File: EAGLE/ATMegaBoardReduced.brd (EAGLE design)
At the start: 55.9 x 50.5 mm, 18 parts, among them IC2 ATMEGA168-20P, IC3 REG1117, X1 49S/18PF

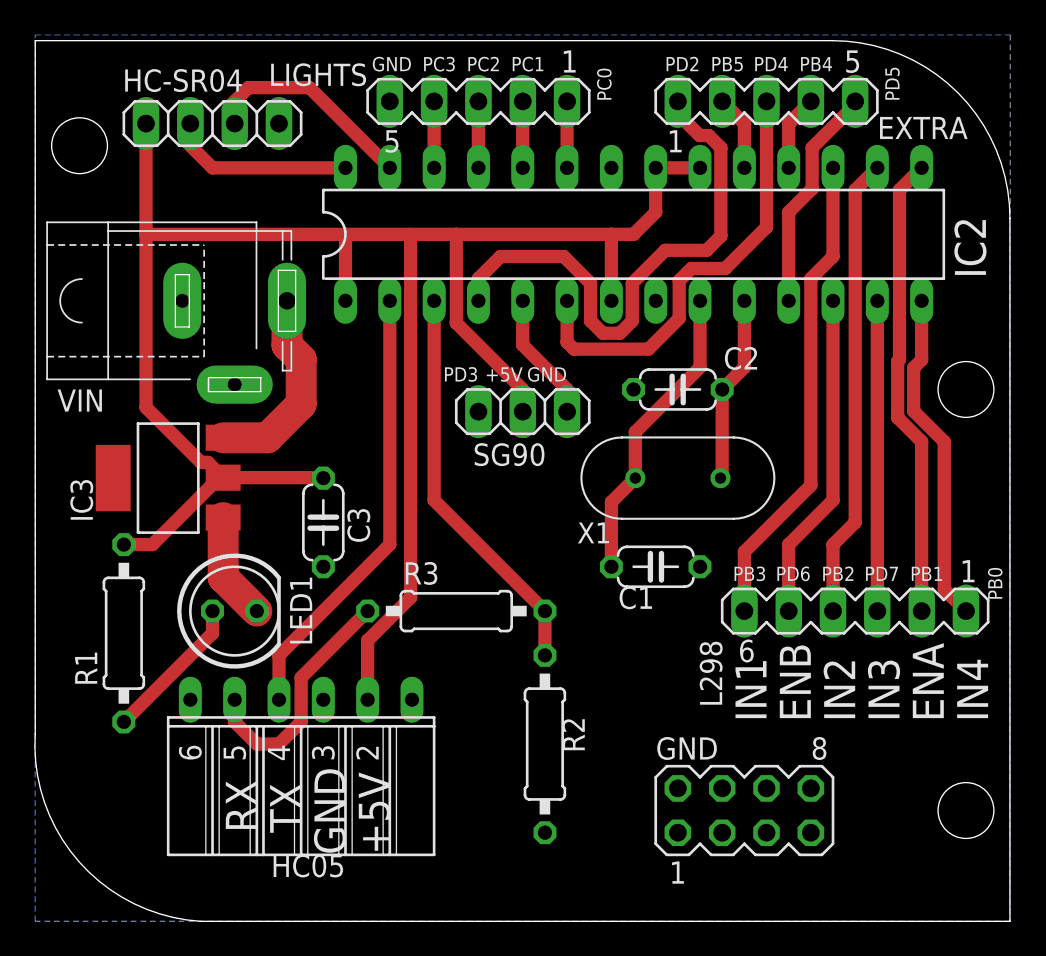
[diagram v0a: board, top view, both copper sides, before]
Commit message: minor board updates
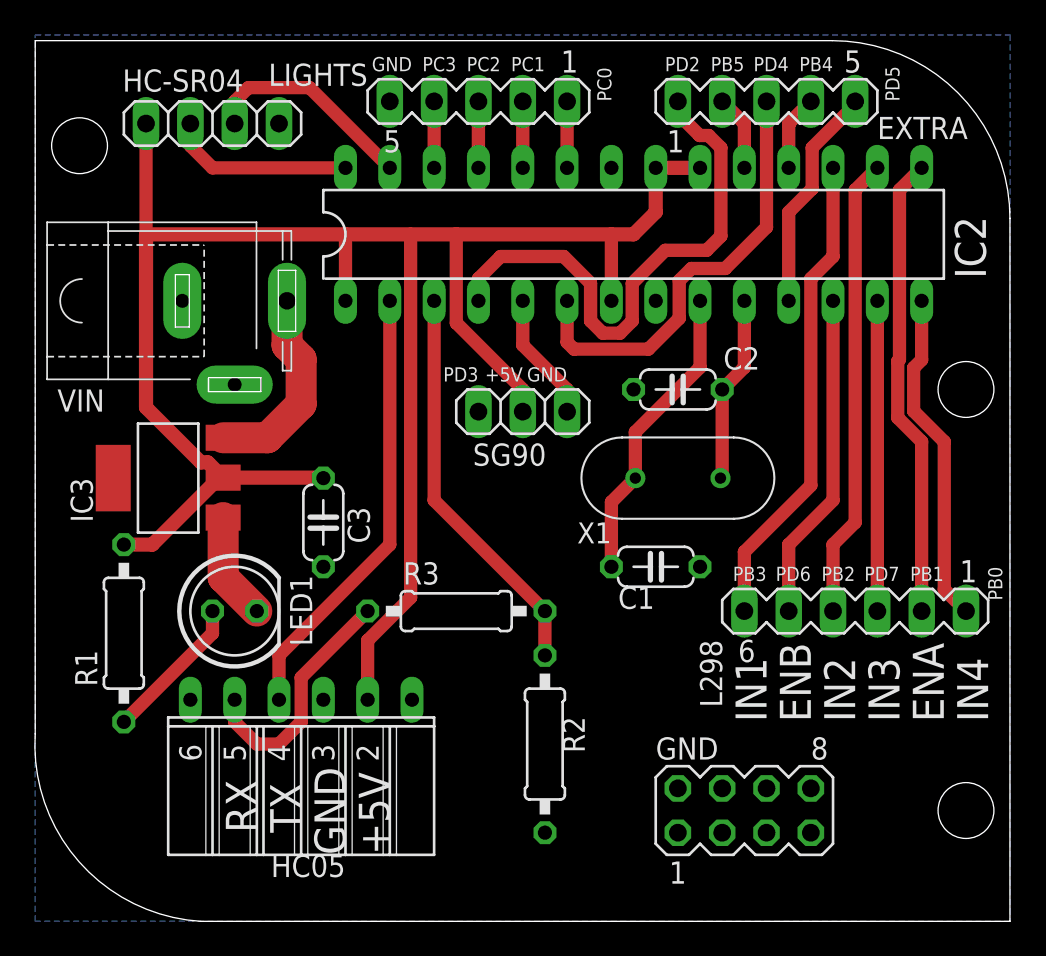
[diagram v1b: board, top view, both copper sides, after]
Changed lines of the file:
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@@
 <drawing>
 <settings>
-<setting alwaysvectorfont="yes"/>
+<setting alwaysvectorfont="no"/>
 <setting verticaltext="up"/>
 </settings>
@@
 <contactref element="HC05" pad="2"/>
 <wire x1="45.72" y1="40.64" x2="45.72" y2="44.45" width="0.762" layer="1"/>
-<wire x1="19.41325625" y1="26.67" x2="23.24865625" y2="30.5054" width="0.762" layer="1"/>
-<wire x1="19.41325625" y1="26.67" x2="17.78" y2="26.67" width="0.762" layer="1"/>
+<wire x1="19.41325625" y1="26.67" x2="23.24865625" y2="30.5054" width="0.8128" layer="1"/>
+<wire x1="19.41325625" y1="26.67" x2="17.78" y2="26.67" width="0.8128" layer="1"/>
 <wire x1="36.83" y1="39.37" x2="36.83" y2="44.45" width="0.762" layer="1"/>
 <wire x1="40.64" y1="34.29" x2="40.64" y2="35.56" width="0.762" layer="1"/>
@@
 <wire x1="34.2138" y1="23.63550625" x2="34.2138" y2="44.3738" width="0.762" layer="1"/>
 <wire x1="29.1846" y1="30.5054" x2="29.21" y2="30.48" width="0.762" layer="1"/>
-<wire x1="23.4696" y1="30.5054" x2="22.5933" y2="31.3817" width="0.762" layer="1"/>
-<wire x1="22.5933" y1="31.3817" x2="22.19275625" y2="31.3817" width="0.762" layer="1"/>
-<wire x1="22.19275625" y1="31.3817" x2="19.05" y2="34.52445625" width="0.762" layer="1"/>
-<wire x1="19.05" y1="34.52445625" x2="19.05" y2="44.45" width="0.762" layer="1"/>
-<wire x1="19.05" y1="44.45" x2="30.48" y2="44.45" width="0.762" layer="1"/>
-<wire x1="30.48" y1="44.45" x2="34.1376" y2="44.45" width="0.762" layer="1"/>
-<wire x1="36.83" y1="44.45" x2="45.72" y2="44.45" width="0.762" layer="1"/>
-<wire x1="45.72" y1="44.45" x2="46.99" y2="44.45" width="0.762" layer="1"/>
-<wire x1="48.26" y1="48.26" x2="50.8" y2="48.26" width="0.762" layer="1"/>
-<wire x1="46.99" y1="44.45" x2="48.26" y2="45.72" width="0.762" layer="1"/>
-<wire x1="48.26" y1="45.72" x2="48.26" y2="48.26" width="0.762" layer="1"/>
+<wire x1="23.4696" y1="30.5054" x2="22.5933" y2="31.3817" width="0.8128" layer="1"/>
+<wire x1="22.5933" y1="31.3817" x2="22.19275625" y2="31.3817" width="0.8128" layer="1"/>
+<wire x1="22.19275625" y1="31.3817" x2="19.05" y2="34.52445625" width="0.8128" layer="1"/>
+<wire x1="19.05" y1="34.52445625" x2="19.05" y2="44.45" width="0.8128" layer="1"/>
+<wire x1="19.05" y1="44.45" x2="30.48" y2="44.45" width="0.8128" layer="1"/>
+<wire x1="30.48" y1="44.45" x2="34.1376" y2="44.45" width="0.8128" layer="1"/>
+<wire x1="36.83" y1="44.45" x2="45.72" y2="44.45" width="0.8128" layer="1"/>
+<wire x1="45.72" y1="44.45" x2="46.99" y2="44.45" width="0.8128" layer="1"/>
+<wire x1="48.26" y1="48.26" x2="50.8" y2="48.26" width="0.8128" layer="1"/>
+<wire x1="46.99" y1="44.45" x2="48.26" y2="45.72" width="0.8128" layer="1"/>
+<wire x1="48.26" y1="45.72" x2="48.26" y2="48.26" width="0.8128" layer="1"/>
 <wire x1="23.24865625" y1="30.5054" x2="23.4696" y2="30.5054" width="0.762" layer="1"/>
-<wire x1="23.4696" y1="30.5054" x2="29.1846" y2="30.5054" width="0.762" layer="1"/>
+<wire x1="23.4696" y1="30.5054" x2="29.1846" y2="30.5054" width="0.8128" layer="1"/>
 <wire x1="34.2138" y1="44.3738" x2="34.1376" y2="44.45" width="0.762" layer="1"/>
 <wire x1="34.2138" y1="44.3738" x2="34.29" y2="44.45" width="0.762" layer="1"/>
-<wire x1="34.29" y1="44.45" x2="36.83" y2="44.45" width="0.762" layer="1"/>
+<wire x1="34.29" y1="44.45" x2="36.83" y2="44.45" width="0.8128" layer="1"/>
 <contactref element="IC2" pad="1"/>
 <wire x1="30.48" y1="40.64" x2="30.48" y2="44.45" width="0.762" layer="1"/>
